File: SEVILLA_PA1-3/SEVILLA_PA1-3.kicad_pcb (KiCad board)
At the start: 2 copper layers, 100 x 50 mm, 15 parts, among them J1 Conn_01x02, SW3 SW_SPST, SW4 SW_SPST, U1 HDSP-7401, U2 PIC16F84A-XXP, U3 HDSP-7401, Y1 4 MHz

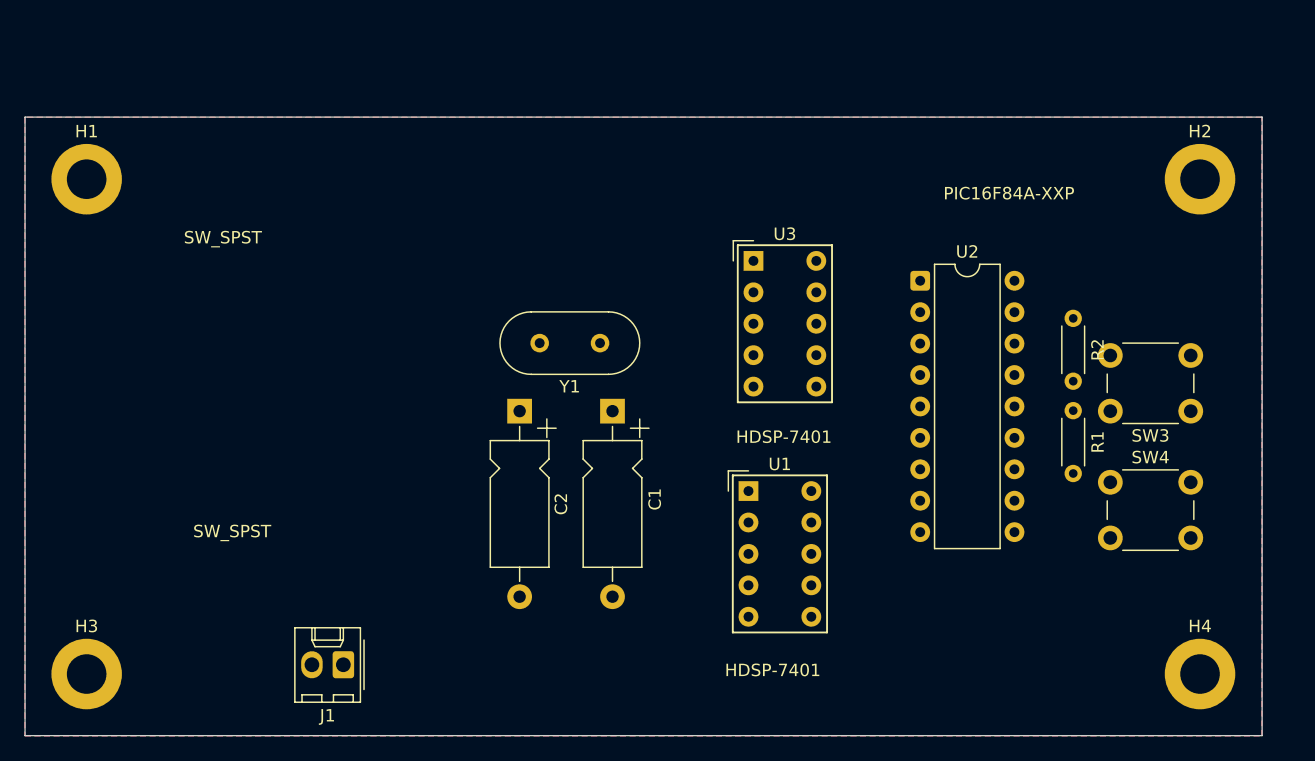
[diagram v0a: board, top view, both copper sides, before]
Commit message: Refactor code structure for improved readability and maintainability
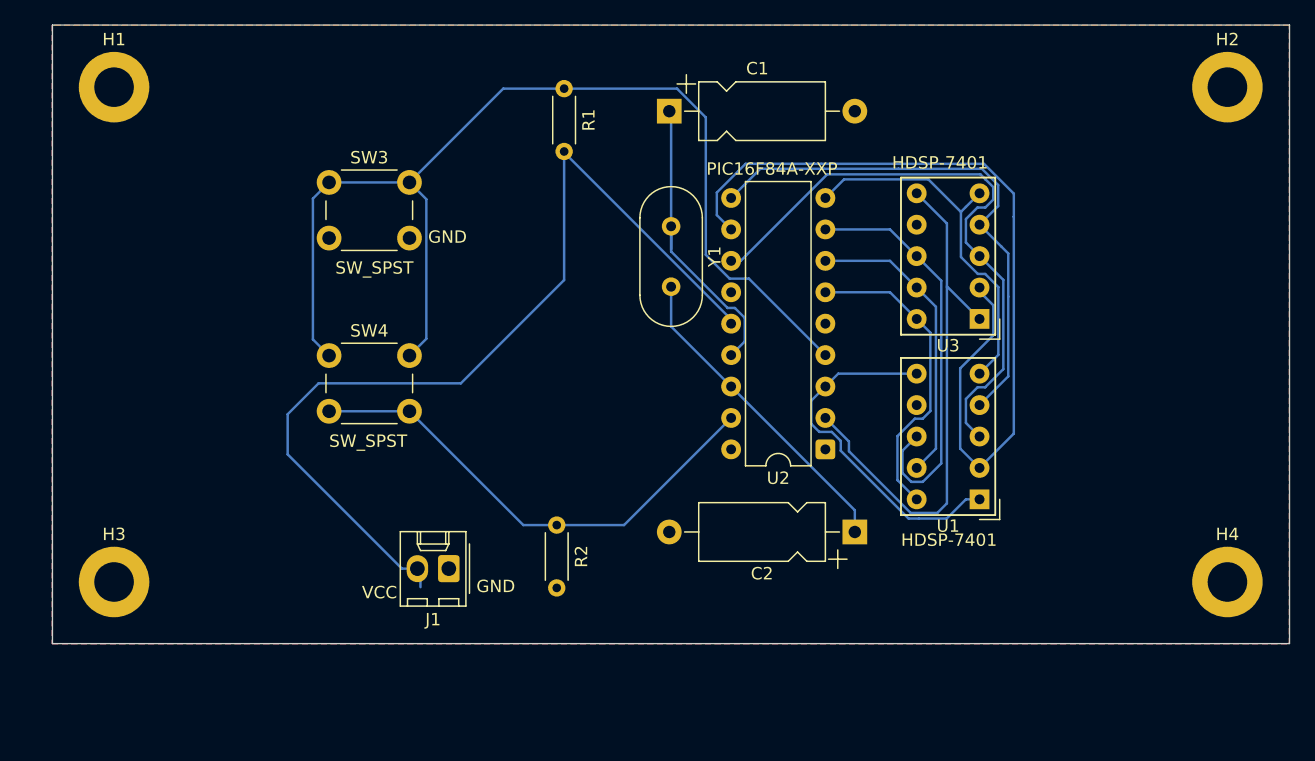
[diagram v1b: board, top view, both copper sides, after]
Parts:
- moved SW3 72.1 mm to (121.1, 74.3), turned to 0 degrees
- moved SW4 64.0 mm to (121.1, 88.3)
- moved R1 48.7 mm to (140.1, 71.8)
- moved R2 45.0 mm to (139.5, 102.0)
- moved C2 28.8 mm to (163.6, 102.5), turned to 180 degrees
- moved C1 24.7 mm to (148.6, 68.5), turned to 0 degrees
- moved U3 18.9 mm to (173.7, 85.3), turned to 180 degrees
- moved U1 18.7 mm to (173.7, 99.9), turned to 180 degrees
- moved U2 15.6 mm to (161.2, 95.8), turned to 180 degrees
- moved J1 11.5 mm to (130.8, 105.5)
- moved Y1 11.1 mm to (148.7, 77.8), turned to -90 degrees
- moved H1 7.76 mm to (103.7, 66.6)
- moved H2 7.76 mm to (193.7, 66.6)
- moved H3 7.76 mm to (103.7, 106.6)
- moved H4 7.76 mm to (193.7, 106.6)
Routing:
- net Net-(SW3-A): track 0.00 -> 88.9 mm
- net VCC: track 0.00 -> 75.5 mm
- net Net-(U1-F): track 0.00 -> 69.5 mm
- net Net-(U1-G): track 0.00 -> 49.3 mm
- net Net-(U2-RA3): track 0.00 -> 43.6 mm
- net Net-(U1-E): track 0.00 -> 43.4 mm
- net Net-(SW4-B): track 0.00 -> 39.9 mm
- net Net-(U1-C): track 0.00 -> 33.3 mm
- net Net-(U1-D): track 0.00 -> 30.1 mm
- net Net-(U2-TOCKI/RA4): track 0.00 -> 29.2 mm
- net Net-(U2-OSC1/CLKIN): track 0.00 -> 26.0 mm
- net Net-(U1-A): track 0.00 -> 25.4 mm
- net Net-(U2-OSC2/CLKOUT): track 0.00 -> 24.7 mm
- net Net-(U1-B): track 0.00 -> 24.1 mm
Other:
- board text added: "GND"
- board text added: "VCC"
